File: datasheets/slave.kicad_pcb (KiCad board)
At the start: 2 copper layers, 71.1 x 50.8 mm, 26 parts, among them J1 Screw_Terminal_1x02, J2 Screw_Terminal_1x03, J3 Screw_Terminal_1x02, Q1 IRFU9024N, Q2 IRFU9024N, Q3 IRFU9024N, U1 PC817, U2 PC817, U3 PC817, U4 nRF24L01, U5 ArduinoNano, U6 KA378R33

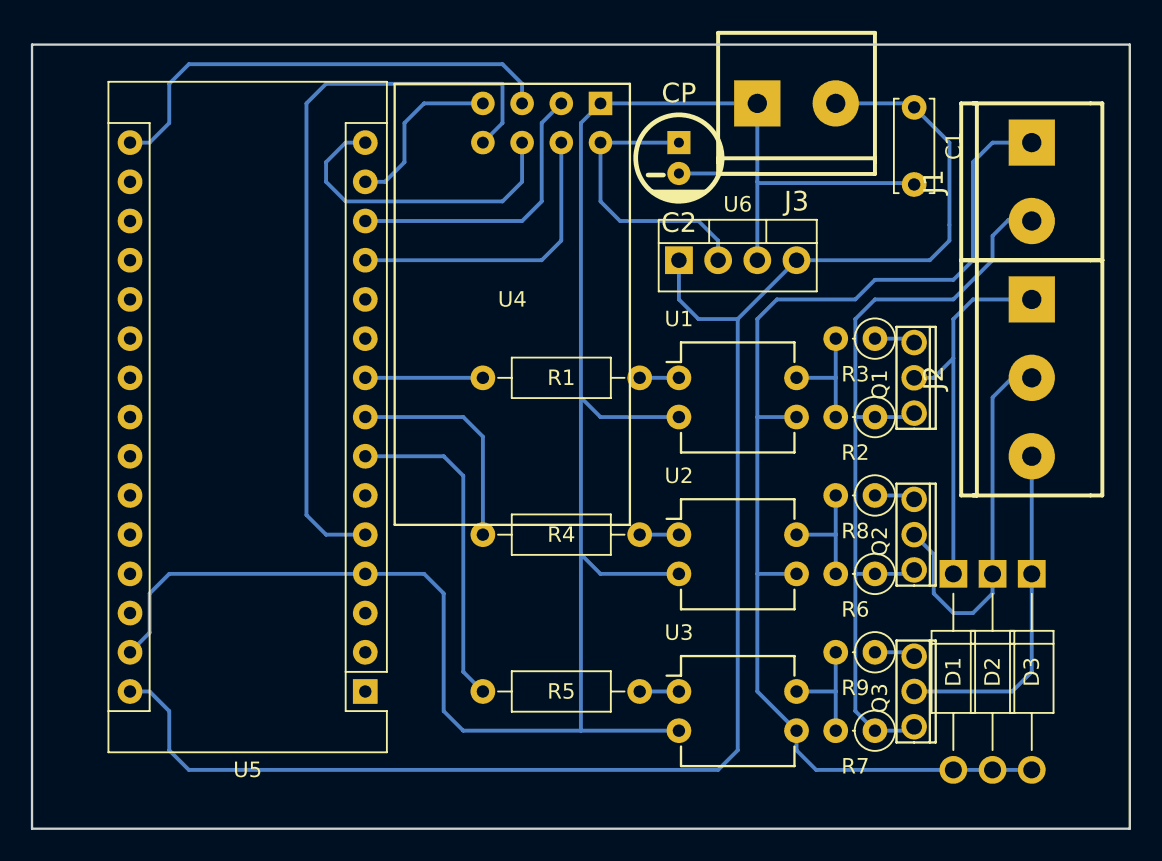
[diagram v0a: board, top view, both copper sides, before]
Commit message: Добавление библиотек компонентов для KiCad.
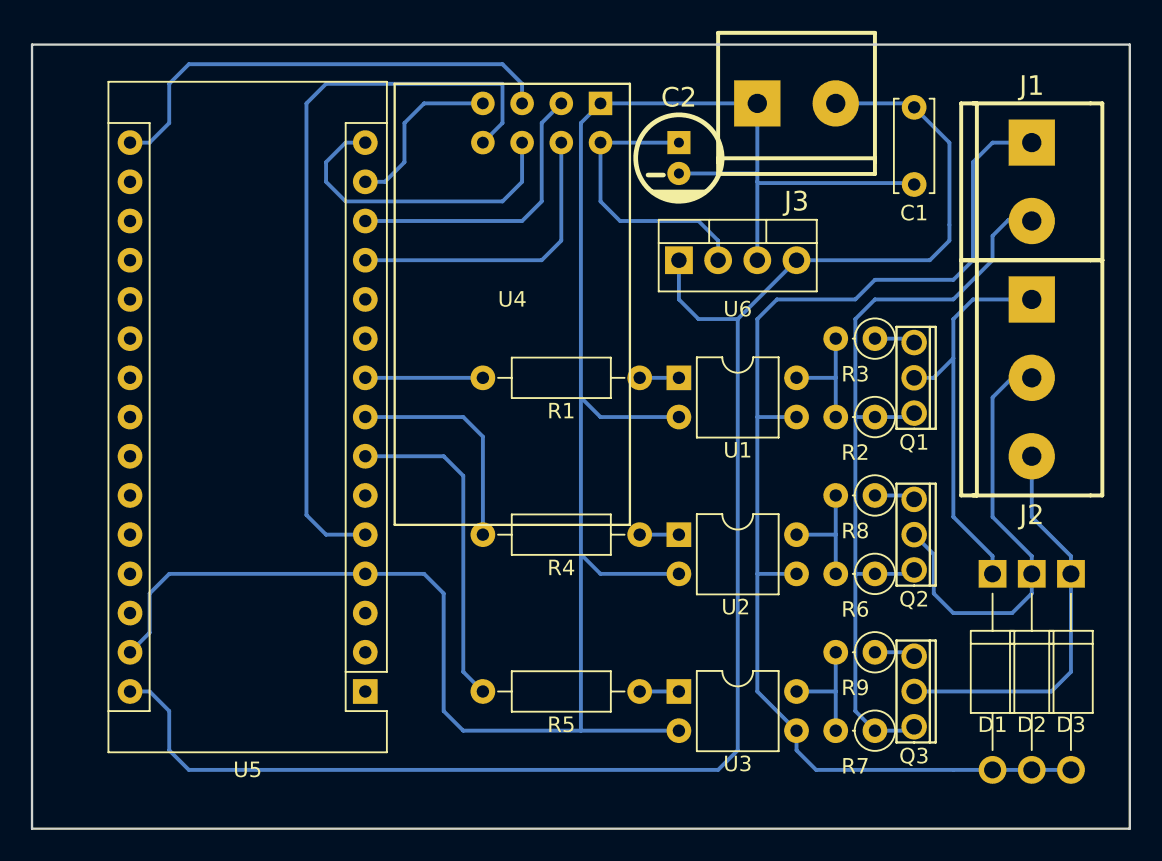
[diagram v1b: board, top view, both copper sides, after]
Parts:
- moved D3 2.54 mm to (251.5, 83.8)
- moved D1 2.54 mm to (246.4, 83.8)
- moved D2 2.54 mm to (248.9, 83.8)
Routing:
- net /OUT_2: track 25.0 -> 28.6 mm
- net /OUT_3: track 22.3 -> 25.7 mm
- net /P_GND: track 76.1 -> 78.6 mm
- net /OUT_1: track 25.2 -> 26.2 mm
